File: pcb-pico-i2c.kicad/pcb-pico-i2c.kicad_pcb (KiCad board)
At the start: 2 copper layers, 13.7 x 20.4 mm, 7 parts, among them J1 Grove, J2 Connector_Pico_I2C, J3 Stemma QT, J4 RUN, J5 3V3_EN, SW1 SW_Push, SW2 SW_Push

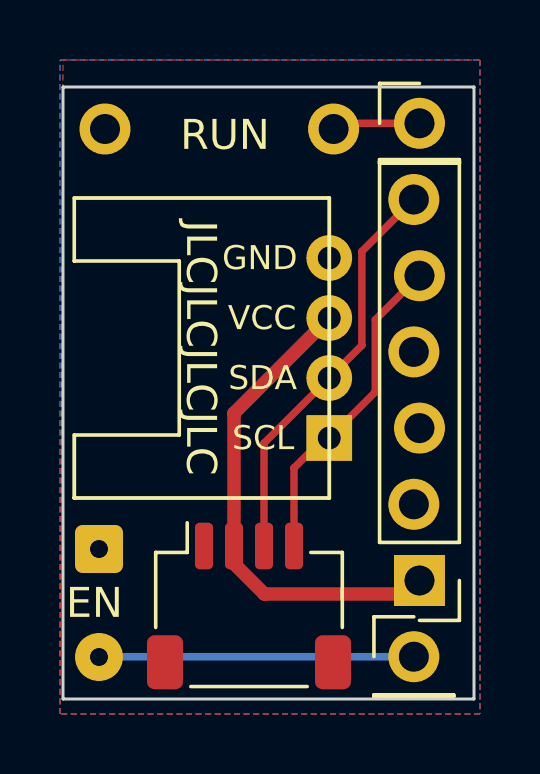
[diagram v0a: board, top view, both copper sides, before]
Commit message: changes for Rev3 of board
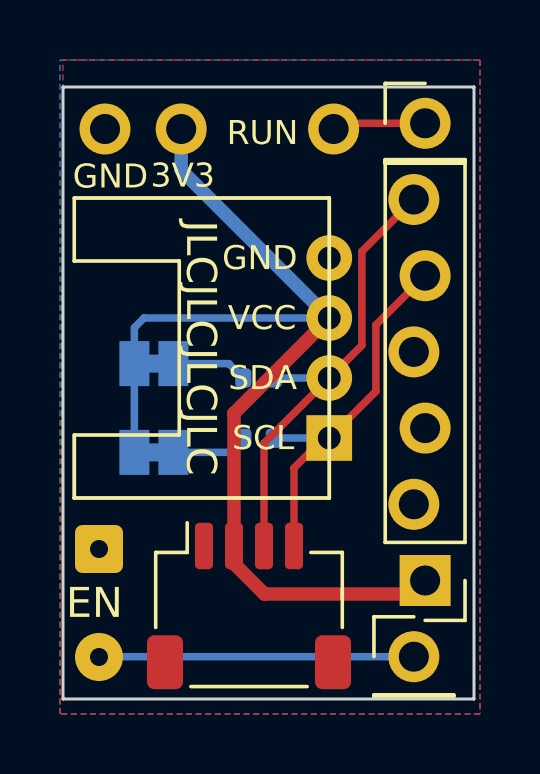
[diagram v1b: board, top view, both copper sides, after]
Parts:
- added J6: 3V3, user:PinHole_1x01, B.Cu at (116.8, 70.3)
- added JP1: SolderJumper_2_Bridged, Jumper:SolderJumper-2_P1.3mm_Bridged_Pad1.0x1.5mm, B.Cu at (115.8, 81.1)
- added JP2: SolderJumper_2_Bridged, Jumper:SolderJumper-2_P1.3mm_Bridged_Pad1.0x1.5mm, B.Cu at (115.8, 78.1)
- added R1: R, Resistor_SMD:R_0402_1005Metric, B.Cu at (119.3, 80.6)
- added R2: R, Resistor_SMD:R_0402_1005Metric, B.Cu at (119.3, 78.6)
- moved J2 0.19 mm to (124.9, 85.3)
- moved J4 0.19 mm to (124.9, 70.1)
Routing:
- net Net-(J1-Pad3): track 16.3 -> 35.4 mm
- net Net-(JP2-Pad2): track 0.00 -> 2.53 mm
- net Net-(JP1-Pad2): track 0.00 -> 2.52 mm
- net Net-(J1-Pad1): track 10.8 -> 12.8 mm
- net Net-(J1-Pad2): track 13.6 -> 15.5 mm
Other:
- board text added: "3V3"
- board text added: "GND"
- board text added: "Rev: 3"
- board text added: "github.com/ bablokb/"
- board text added: "pcb-pico-i2c"
- board text removed: "Rev: 2"
- board text removed: "https://github.com/bablokb/ pcb-pico-i2c"
